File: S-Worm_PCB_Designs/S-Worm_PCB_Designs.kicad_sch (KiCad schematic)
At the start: 10 parts

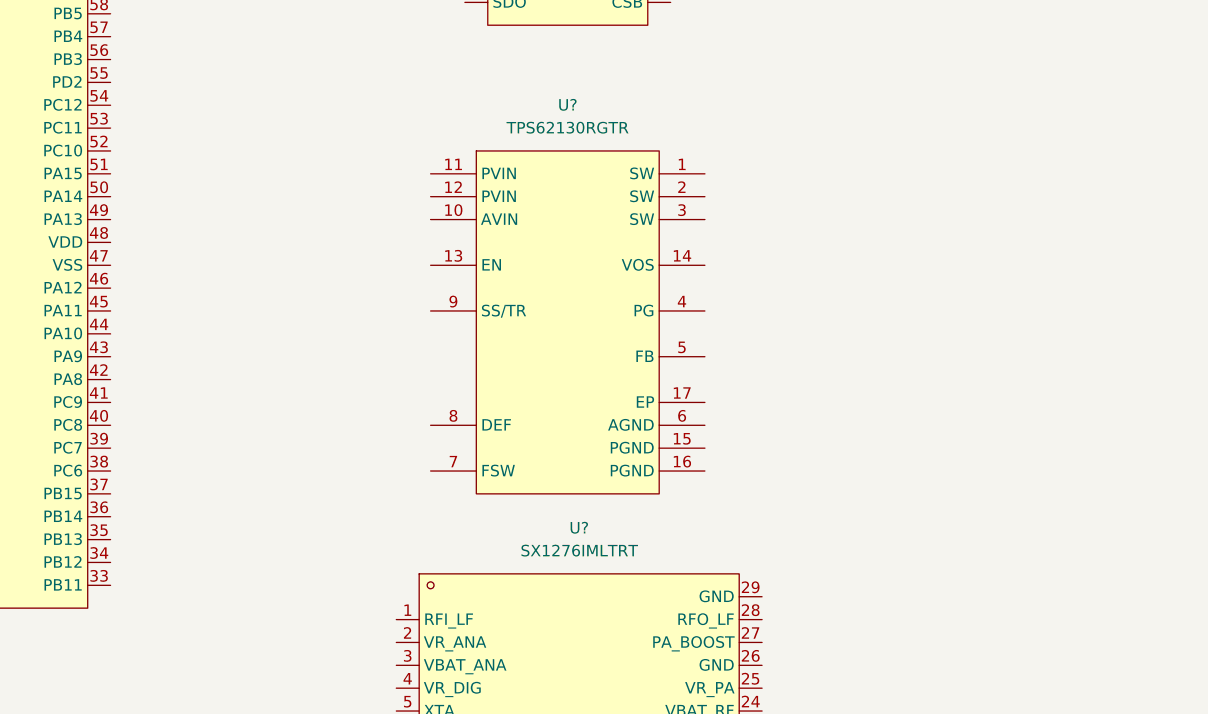
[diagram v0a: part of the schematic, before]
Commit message: mag
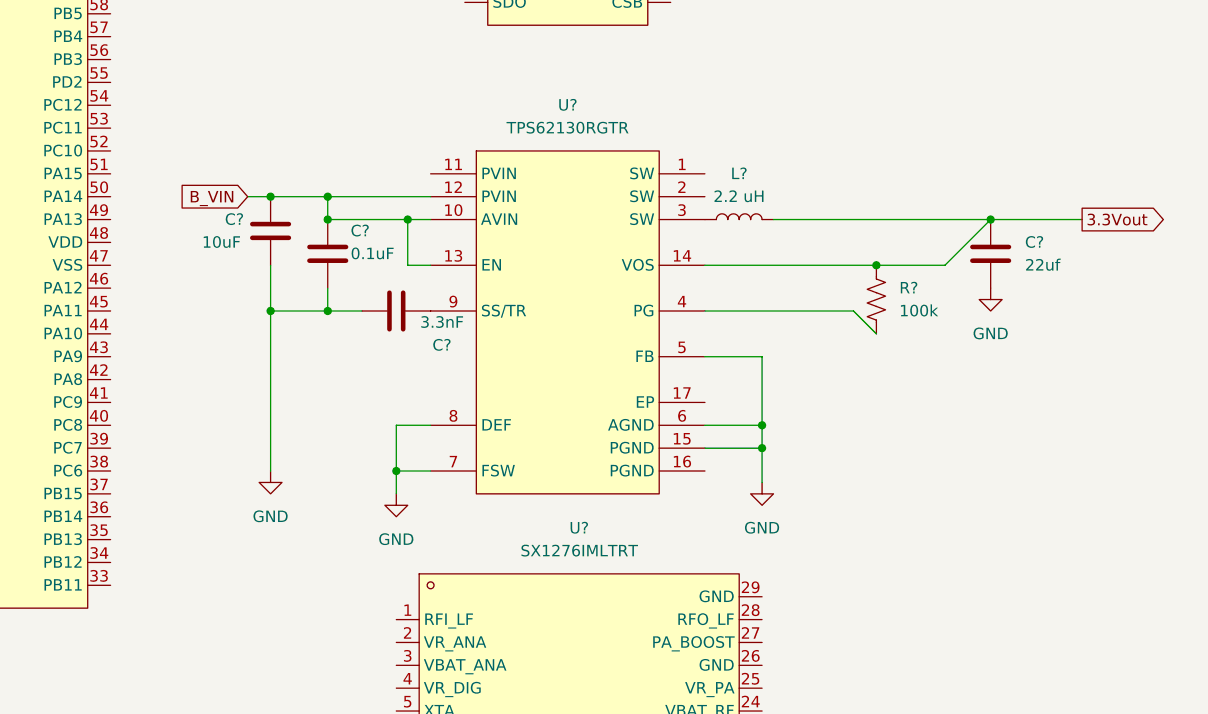
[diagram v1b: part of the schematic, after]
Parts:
- added C?: 10uF, symbol Device:C
- added C?: 0.1uF, symbol Device:C
- added C?: 22uf, symbol Device:C
- added C?: 3.3nF, symbol Device:C
- added L?: 2.2 uH, symbol Device:L
- added R?: 100k, symbol Device:R_US
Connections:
- net B_VIN: now reaches U?.10 (AVIN)
- net B_VIN: now also U?.12 (PVIN), U?.13 (EN), C?.1, C?.1
- net 3.3Vout: now reaches U?.14 (VOS)
- net 3.3Vout: now also C?.1, L?.2, R?.1
- net GND: now reaches U?.15 (PGND)
- net GND: now also U?.5 (FB), U?.6 (AGND), U?.7 (FSW), U?.8 (DEF), C?.2, C?.2, C?.2, C?.2
- net at U?.3 (SW): now also L?.1
- net at U?.4 (PG): now also R?.2
- net at U?.9 (SS/TR): now also C?.1
